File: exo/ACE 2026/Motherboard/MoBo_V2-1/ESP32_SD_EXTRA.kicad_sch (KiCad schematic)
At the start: 9 parts, among them J601 Conn_02x10_Counter_Clockwise, J602 Micro_SD_Card

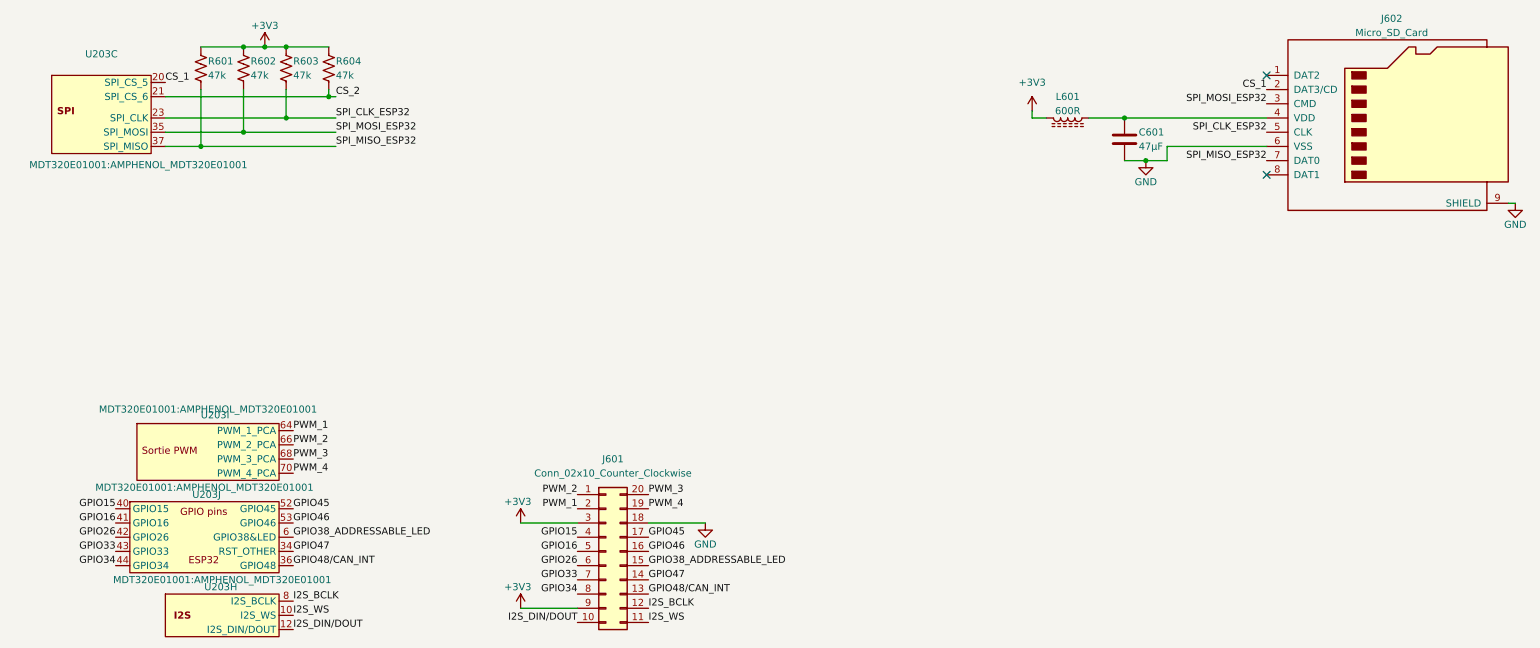
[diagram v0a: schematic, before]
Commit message: Pushing changed files
multiple correctiosn done especially a new Mobo
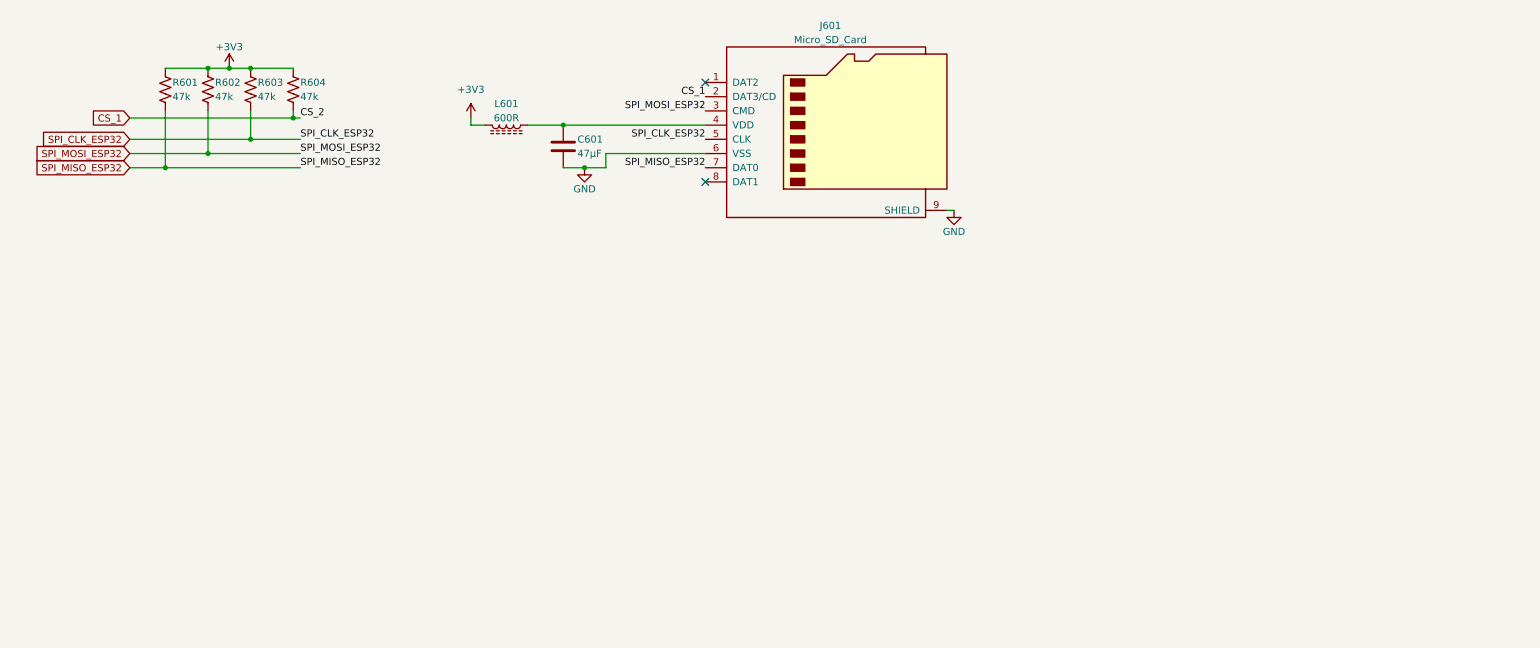
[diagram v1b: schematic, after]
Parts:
- removed J601: Conn_02x10_Counter_Clockwise, Connector_PinSocket_2.54mm:PinSocket_2x10_P2.54mm_Vertical_SMD, symbol Connector_Generic:Conn_02x10_Counter_Clockwise
- removed U203: ~, MDT320E01001:AMPHENOL_MDT320E01001, symbol connecteur_m2_key_E:connecteur_SOM_ESP32_V2
- C601: footprint Capacitor_SMD:C_1206_3216Metric_Pad1.33x1.80mm_HandSolder -> Capacitor_SMD:C_0805_2012Metric_Pad1.18x1.45mm_HandSolder
- R601, R602, R603, R604: footprint Resistor_SMD:R_0603_1608Metric_Pad0.98x0.95mm_HandSolder -> Resistor_SMD:R_0805_2012Metric_Pad1.20x1.40mm_HandSolder
- renumbered J602 to J601
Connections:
- net CS_2 is gone; now on net CS_1: R604.2
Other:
- moved on the sheet: C601, J601, L601, R601, R602, R603, R604
